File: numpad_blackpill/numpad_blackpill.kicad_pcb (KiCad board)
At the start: 2 copper layers, 51 parts, among them SW1 SW_Push, SW10 SW_Push, SW11 SW_Push, SW12 SW_Push, SW13 SW_Push, SW14 SW_Push, SW15 SW_Push, SW16 SW_Push, SW17 SW_Push, SW18 SW_Push, SW19 SW_Push, SW2 SW_Push, SW20 SW_Push, SW21 SW_Push, SW22 SW_Push, SW23 SW_Push, SW24 SW_Push, SW25 SW_Push, SW3 SW_Push, SW4 SW_Push, SW5 SW_Push, SW6 SW_Push, SW7 SW_Push, SW8 SW_Push, SW9 SW_Push, U1 YAAJ_BlackPill

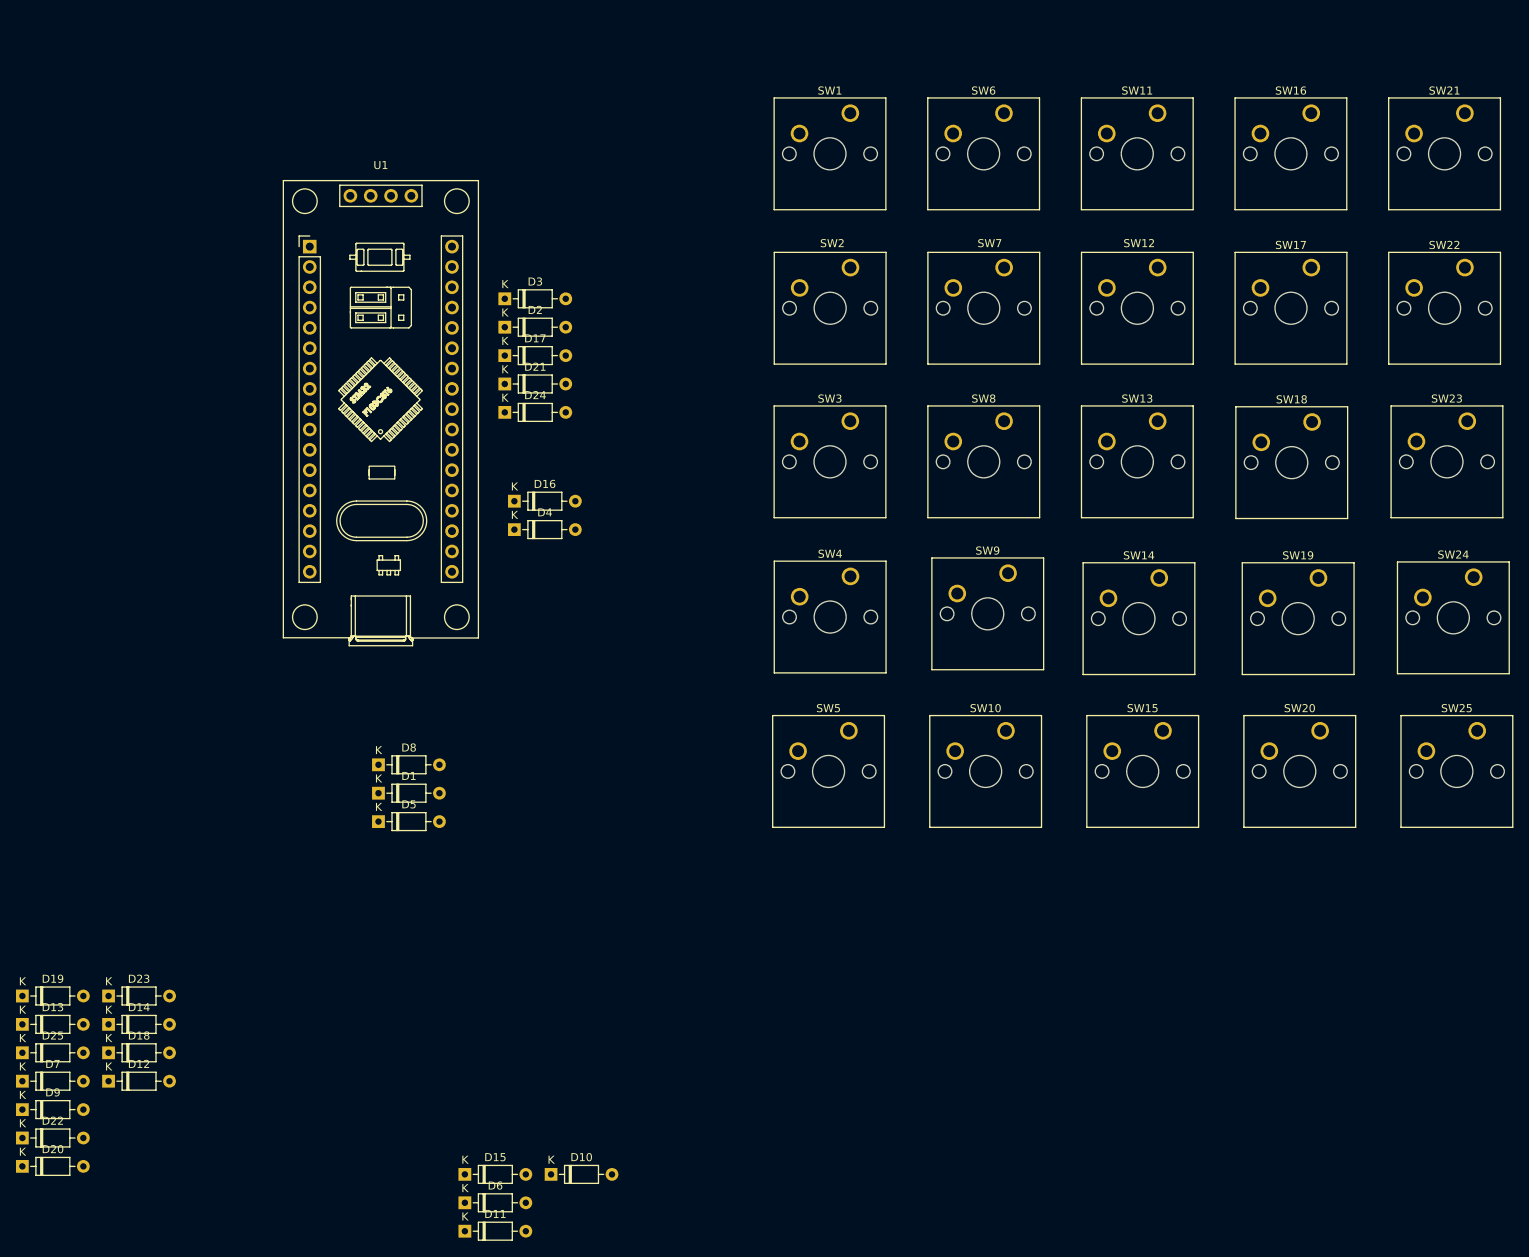
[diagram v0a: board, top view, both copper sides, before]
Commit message: finished basic numpad with blackpill
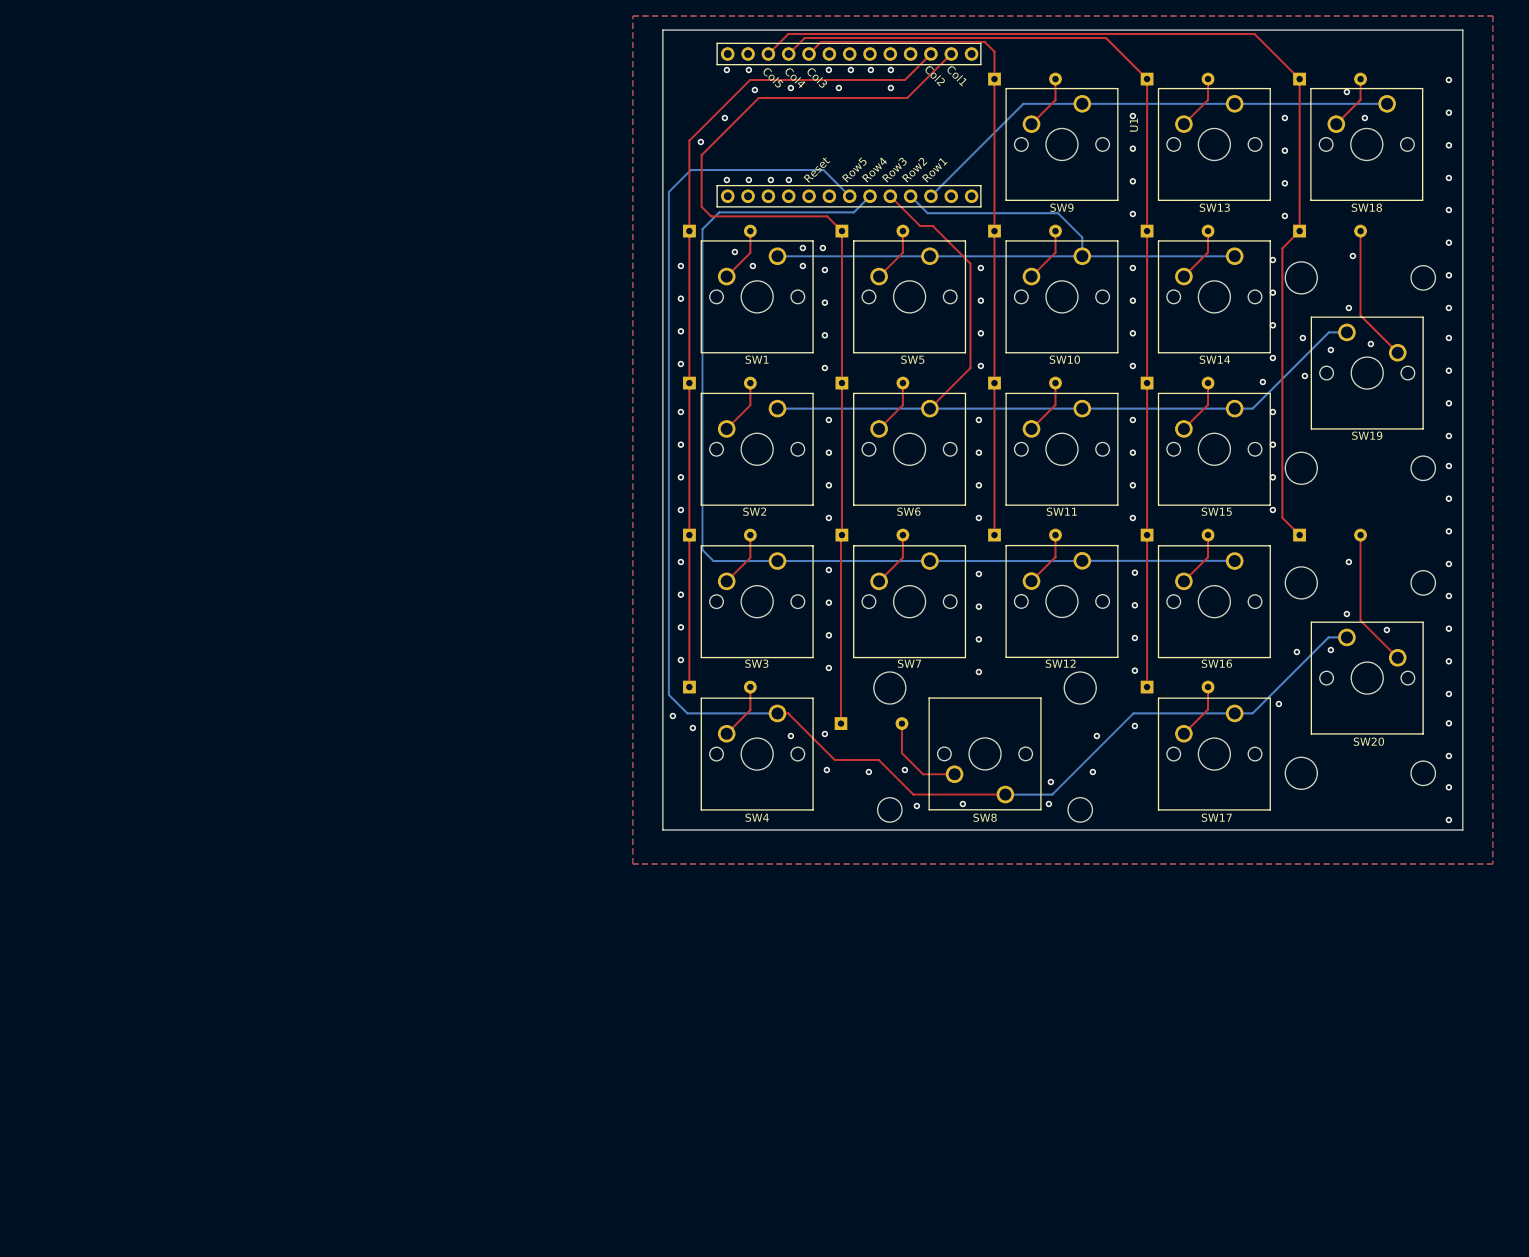
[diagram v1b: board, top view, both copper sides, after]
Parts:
- removed the D1 at (57.7, 114.4)
- removed the D15 at (68.5, 162.1)
- removed the D16 at (74.7, 77.9)
- removed D22, D24: 1N4148, Diode_THT:D_DO-35_SOD27_P7.62mm_Horizontal
- removed the D6 at (68.5, 165.6)
- removed the SW1 at (116.7, 29.4)
- removed the SW15 at (155.8, 106.6)
- removed SW22, SW24, SW25: SW_Push, Button_Switch_Keyboard:SW_Cherry_MX_1.00u_PCB
- removed the SW6 at (135.9, 29.4)
- added D13: 1N4148, Diode_THT:D_DO-35_SOD27_P7.62mm_Horizontal, B.Cu at (153.8, 25.1)
- added SW20: SW_Push, Button_Switch_Keyboard:SW_Cherry_MX_2.00u_Vertical_PCB, B.Cu at (178.8, 94.9)
- D1: renamed from D2; moved to B.Cu
- D10: renamed from D12; moved to B.Cu
- D11: renamed from D13; moved to B.Cu
- D12: renamed from D14; moved to B.Cu
- D14: renamed from D17; moved to B.Cu
- D15: renamed from D18; moved to B.Cu
- D16: renamed from D19; moved to B.Cu
- D17: renamed from D20; moved to B.Cu
- D18: renamed from D21; moved to B.Cu
- D19: renamed from D23; moved to B.Cu
- D2: renamed from D3; moved to B.Cu
- D20: renamed from D25; moved to B.Cu
- D3: renamed from D4; moved to B.Cu
- D4: renamed from D5; moved to B.Cu
- D5: renamed from D7; moved to B.Cu
- D6: renamed from D8; moved to B.Cu
- D7: renamed from D9; moved to B.Cu
- D8: renamed from D10; moved to B.Cu
- D9: renamed from D11; moved to B.Cu
- SW19: renamed from SW23; footprint Button_Switch_Keyboard:SW_Cherry_MX_1.00u_PCB -> Button_Switch_Keyboard:SW_Cherry_MX_2.00u_Vertical_PCB; moved to B.Cu
- SW8: renamed from SW10; footprint Button_Switch_Keyboard:SW_Cherry_MX_1.00u_PCB -> Button_Switch_Keyboard:SW_Cherry_MX_2.00u_PCB; moved to B.Cu
- U1: value YAAJ_BlackPill -> YAAJ_BlackPill_Part_Like_SWD_Breakout; footprint Kicad-STM32-master:YAAJ_BlackPill_SWD_1 -> Kicad-STM32-master:YAAJ_BlackPill_SWD_3
- moved D19 176.9 mm to (172.8, 44.1)
- moved D20 172.3 mm to (172.8, 82.1)
- moved D9 158.5 mm to (134.7, 25.1)
- moved D15 154.5 mm to (153.8, 63.1)
- moved D10 153.5 mm to (134.7, 44.1)
- moved D17 152.8 mm to (153.8, 101.1)
- moved D16 151.9 mm to (153.8, 82.1)
- moved D5 147.6 mm to (115.6, 44.1)
- moved D11 145.6 mm to (134.7, 63.1)
- moved D12 126.5 mm to (134.7, 82.1)
- moved D7 125.1 mm to (115.6, 82.1)
- moved D18 106.4 mm to (172.8, 25.1)
- moved U1 96.0 mm to (142.0, 22.0), turned to -90 degrees
- moved D14 81.8 mm to (153.8, 44.1)
- moved D6 75.1 mm to (115.6, 63.1)
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- renumbered SW2 to SW1, SW12 to SW10, SW13 to SW11, SW14 to SW12, SW16 to SW13, SW17 to SW14, SW18 to SW15, SW19 to SW16, SW20 to SW17, SW21 to SW18, SW3 to SW2, SW4 to SW3, SW5 to SW4, SW7 to SW5, SW8 to SW6, SW9 to SW7, SW11 to SW9
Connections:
- U1 pad 13: Col1 -> Col3
- U1 pad 14: Col2 -> Col4
- U1 pad 15: Col3 -> Col5
- U1 pad 17: unconnected-(U1-Pad17) -> GND
- U1 pad 18: unconnected-(U1-Pad18) -> GND
- U1 pad 19: Col4 -> unconnected-(U1-Pad19)
- U1 pad 20: Col5 -> unconnected-(U1-Pad20)
- U1 pad 24: Row1 -> Row5
- U1 pad 25: Row2 -> Row4
- U1 pad 27: Row4 -> Row2
- U1 pad 28: Row5 -> Row1
- U1 pad 6: unconnected-(U1-Pad6) -> Col2
- U1 pad 7: unconnected-(U1-Pad7) -> Col1
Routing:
- net Row5: track 0.00 -> 186.0 mm
- net Row4: track 0.00 -> 129.9 mm
- net Col5: track 0.00 -> 128.6 mm
- net Col4: track 0.00 -> 123.7 mm
- net Col2: track 0.00 -> 123.3 mm
- net Row3: track 0.00 -> 109.2 mm
- net Col1: track 0.00 -> 103.0 mm
- net Col3: track 0.00 -> 84.7 mm
- net Row2: track 0.00 -> 83.1 mm
- net Row1: track 0.00 -> 61.8 mm
- net Net-(D20-Pad2): track 0.00 -> 17.3 mm
- net Net-(D19-Pad2): track 0.00 -> 17.1 mm
- net Net-(D8-Pad2): track 0.00 -> 11.4 mm
- net Net-(D17-Pad2): track 0.00 -> 7.08 mm
- net Net-(D4-Pad2): track 0.00 -> 7.06 mm
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- added copper zone on B.Cu, net GND
- added copper zone on F.Cu, net GND
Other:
- board outline added: 100 x 100 mm
- board text added: "Col1"
- board text added: "Col2"
- board text added: "Col3"
- board text added: "Col4"
- board text added: "Col5"
- board text added: "Reset"
- board text added: "Row1"
- board text added: "Row2"
- board text added: "Row3"
- board text added: "Row4"
- board text added: "Row5"
